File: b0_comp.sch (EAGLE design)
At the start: 267 parts, among them IC1 КР1006ВИ1(NE555), IC3 LM358D, IC4 78L09F, IC6 MEGA8-AI, IC7 74121N, IC8 4030N, IC9 LM324D, T1P T90, -26 MicroMetals Yellow-W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

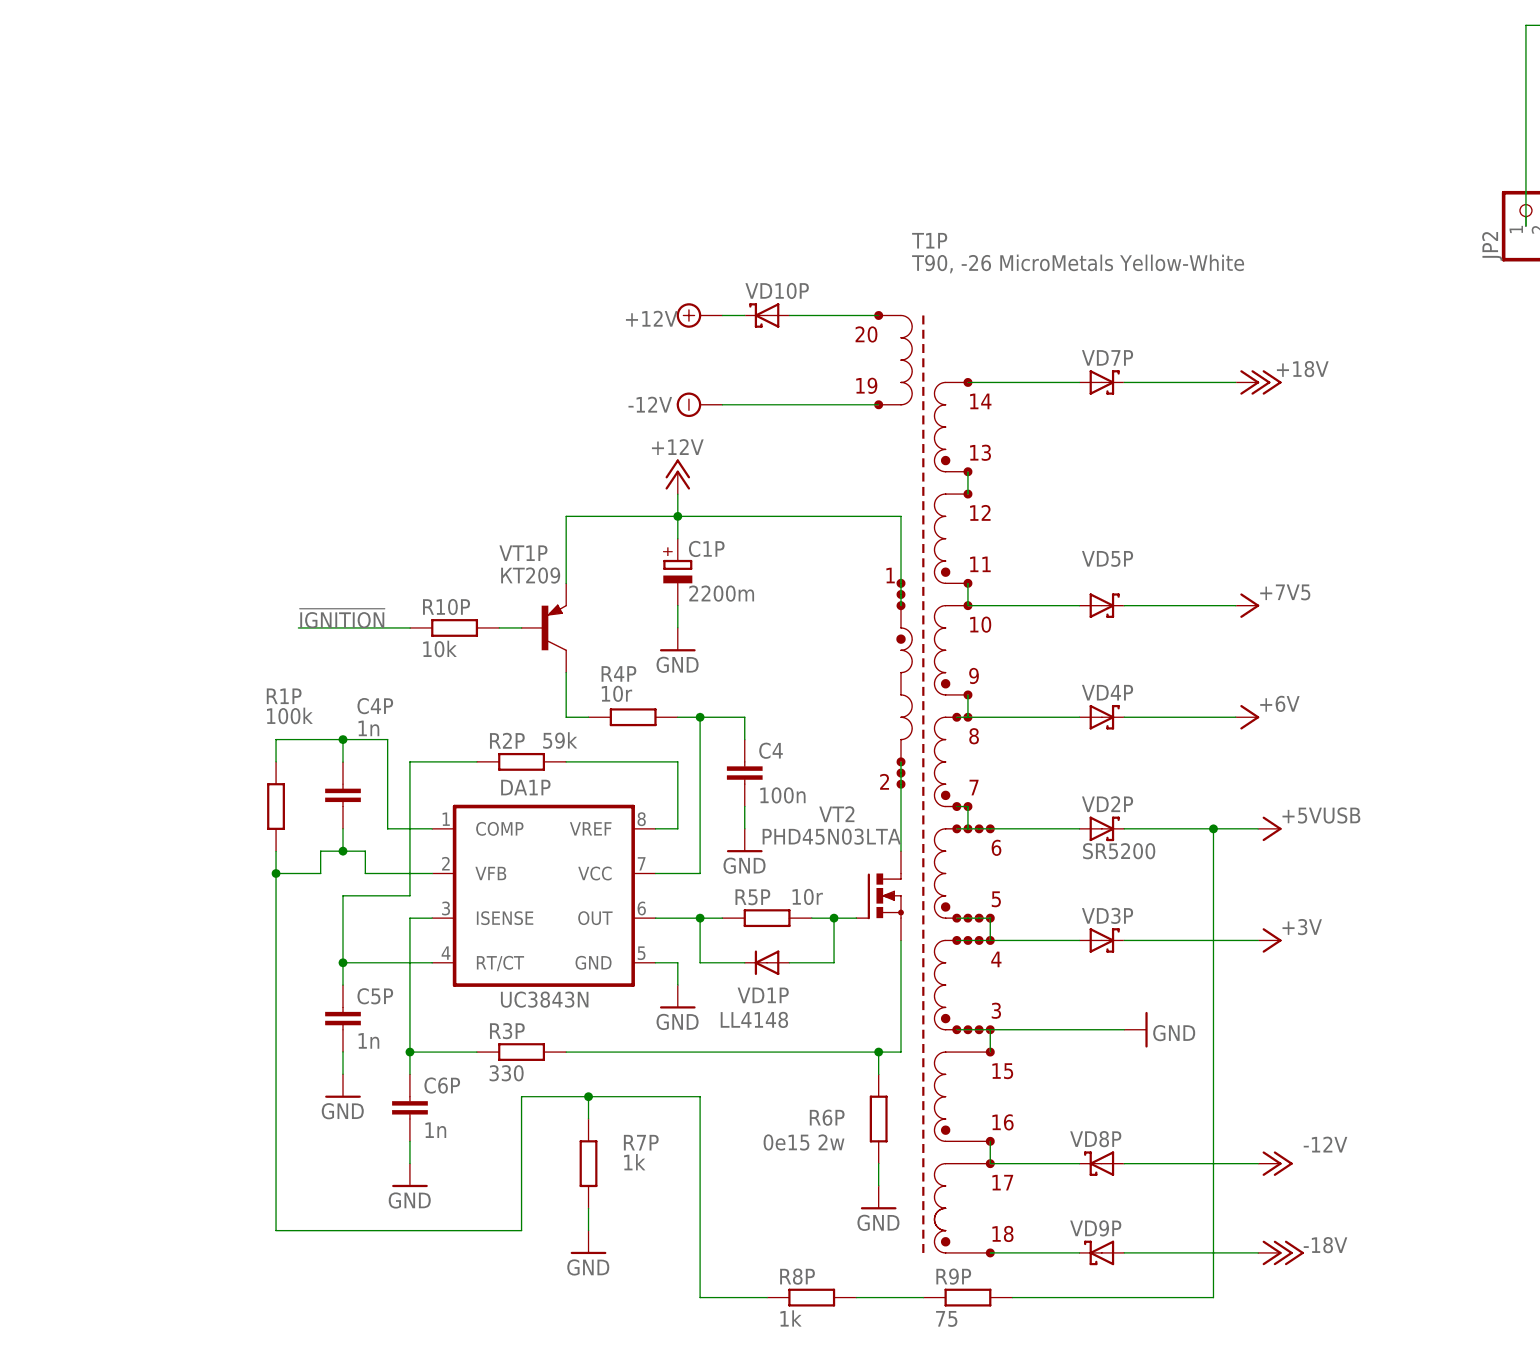
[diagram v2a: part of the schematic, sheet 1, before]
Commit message: .
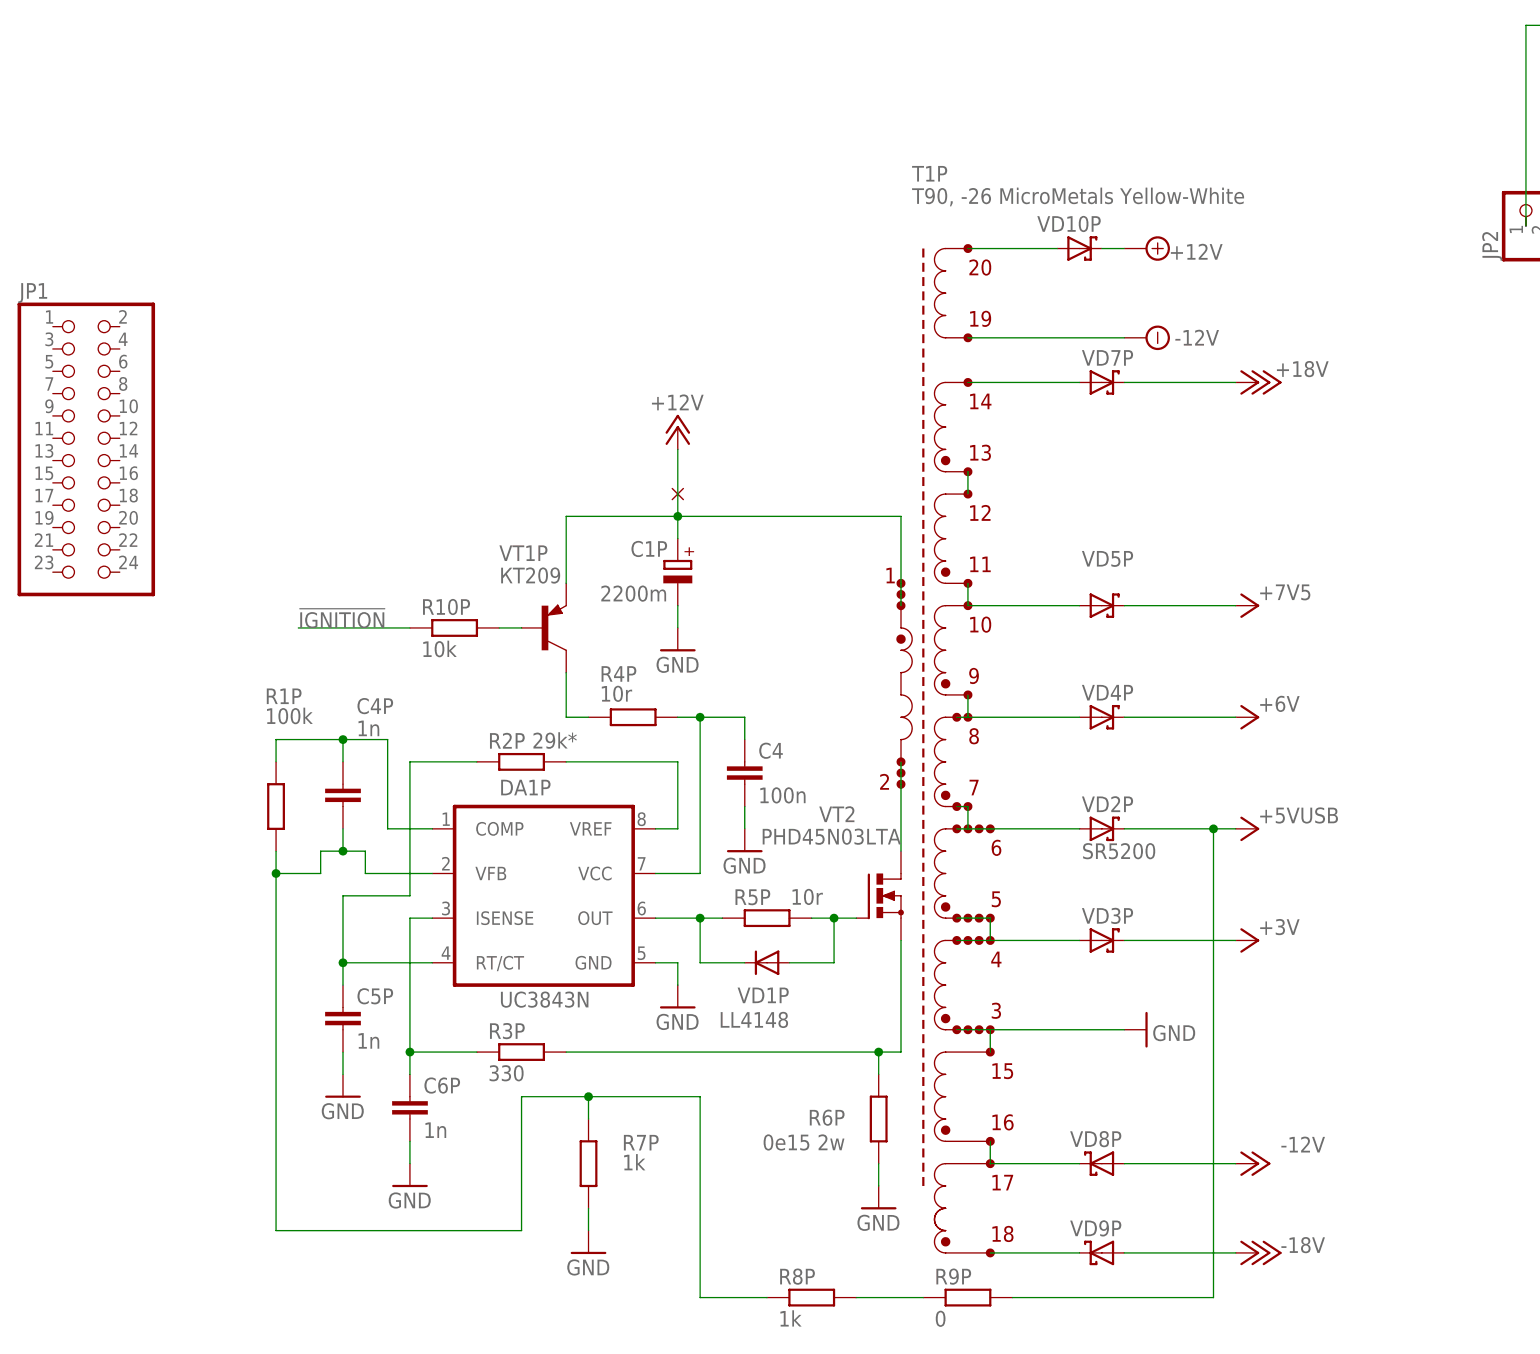
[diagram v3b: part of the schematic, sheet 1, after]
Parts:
- removed U$25: T_PIN_NONAME, b0f:T_PIN_NONAME
- added JP1: (no value), Разъёмы штырьковые 2.54мм:PINHD-2X12
- added U$38: T_PIN_NONAME, b0f:T_PIN_NONAME
- R2P: value 59k -> 29k*
- R9P: value 75 -> 0
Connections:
- net +12V: now also U$38.TNN1; no longer U$23.TNN1
- net N$24: now also U$23.TNN1; no longer U$25.TNN1
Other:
- note added: "5.1v"
- note added: "75*"
- moved on the sheet: 19, 20, C1P, T1P, VD10P

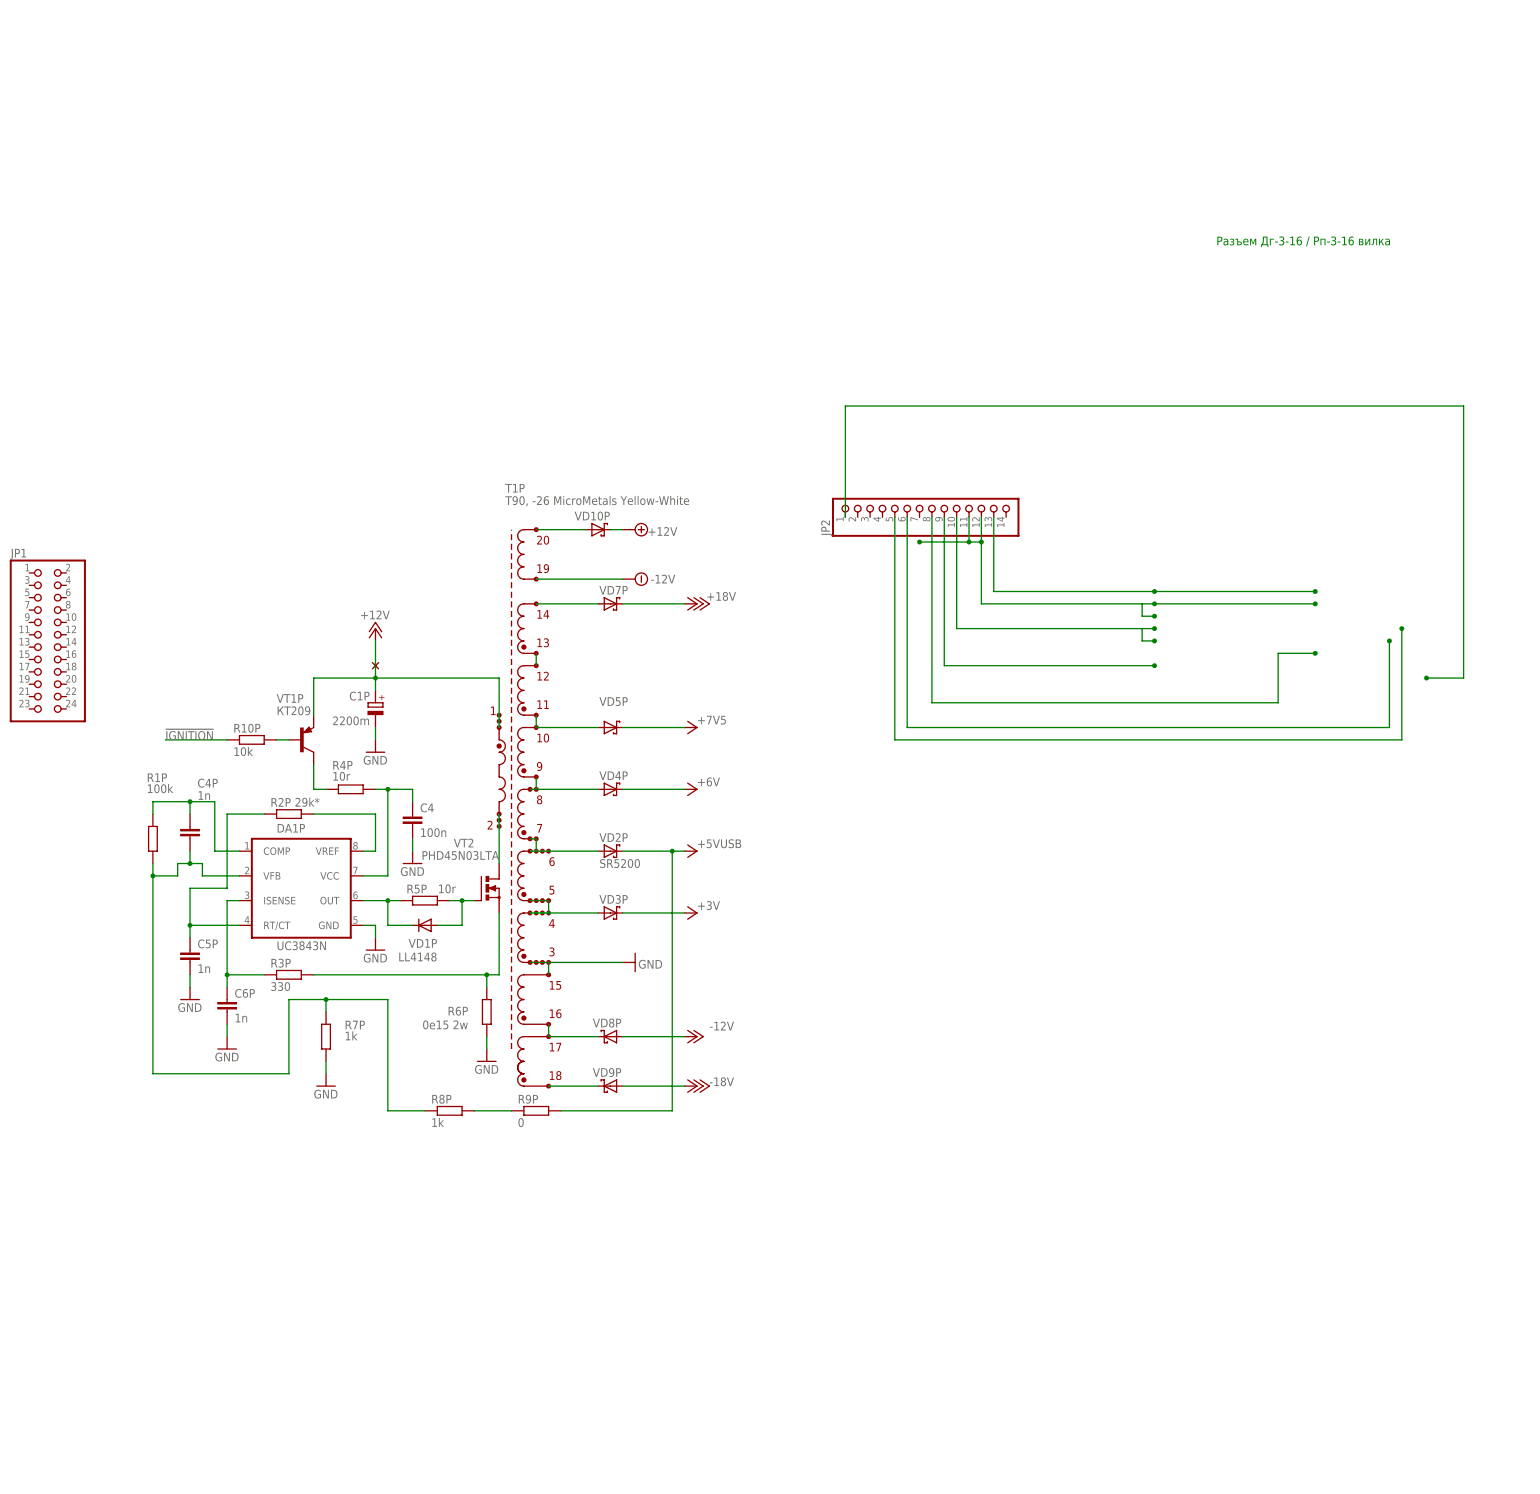
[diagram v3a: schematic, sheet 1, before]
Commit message: .
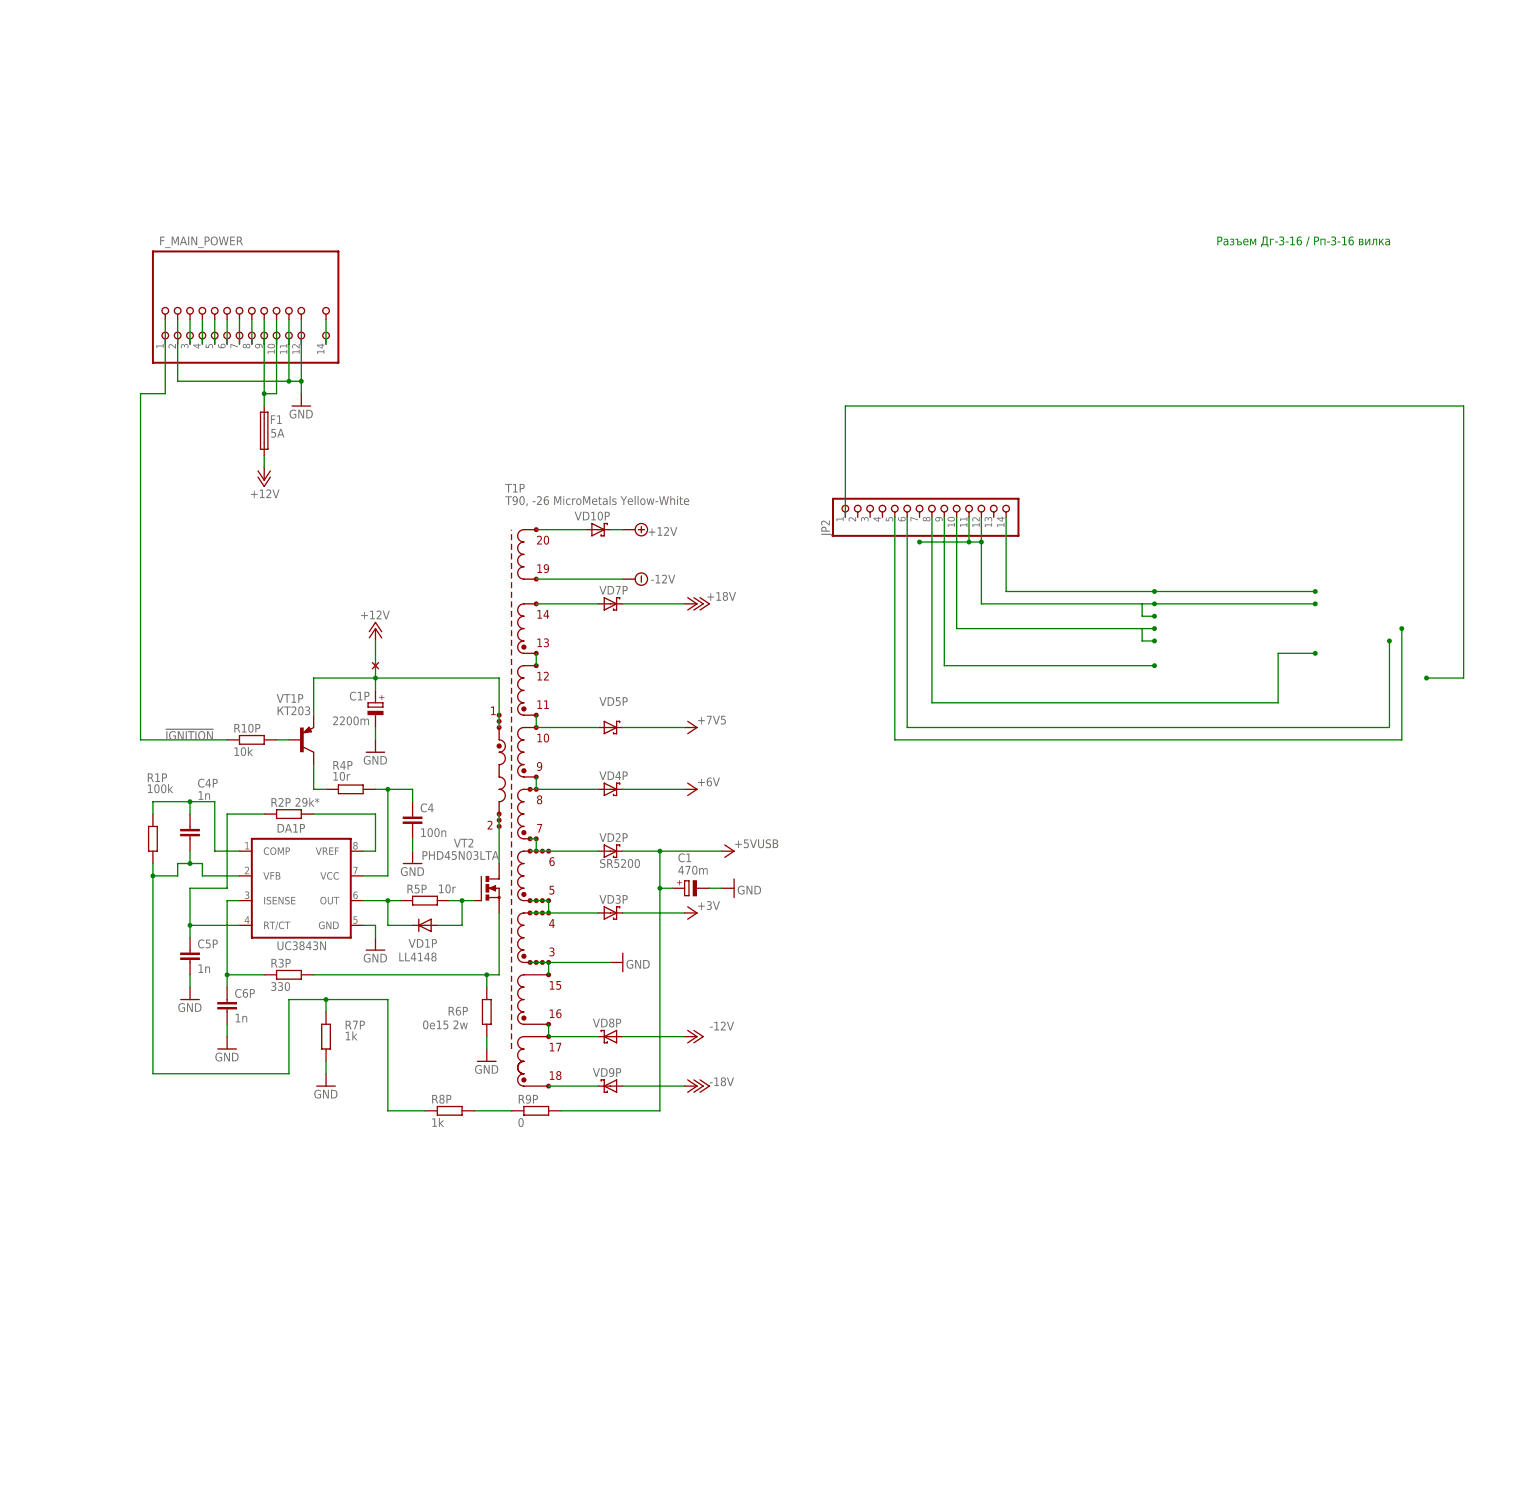
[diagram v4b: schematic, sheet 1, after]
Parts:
- removed JP1: (no value), Разъёмы штырьковые 2.54мм:PINHD-2X12
- added C1: 470m, rcl:CPOL-EUE5-10.5
- added F1: 5A, fuse:FUSESH22,5
- added F_MAIN_POWER: (no value), b0f:PINHD-2X14
- VT1P: value КТ209 -> КТ203; device m_transistor:BJT_PNP_TO-92_ECB -> m_transistor:BJT_PNP_TO18_EBC
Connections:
- new net N$167: F_MAIN_POWER.5, F_MAIN_POWER.6
- new net N$169: F_MAIN_POWER.7, F_MAIN_POWER.8
- new net N$170: F_MAIN_POWER.10, F_MAIN_POWER.9
- new net N$171: F_MAIN_POWER.11, F_MAIN_POWER.12
- new net N$173: F_MAIN_POWER.13, F_MAIN_POWER.14
- new net N$174: F_MAIN_POWER.15, F_MAIN_POWER.16
- new net N$177: F1.2, F_MAIN_POWER.17, F_MAIN_POWER.18, F_MAIN_POWER.19, F_MAIN_POWER.20
- new net N$182: F_MAIN_POWER.27, F_MAIN_POWER.28
- net !IGNITION: now also F_MAIN_POWER.1, F_MAIN_POWER.2
- net +12V: now also F1.1
- net +5VUSB: now also C1.+
- net GND: now also C1.-, F_MAIN_POWER.21, F_MAIN_POWER.22, F_MAIN_POWER.23, F_MAIN_POWER.24, F_MAIN_POWER.3, F_MAIN_POWER.4
- net N$140: now also JP2.14; no longer JP2.13
